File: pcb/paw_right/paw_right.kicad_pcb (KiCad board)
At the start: 2 copper layers, 141.8 x 96 mm, 44 parts, among them U1 Nice_Nano_V2

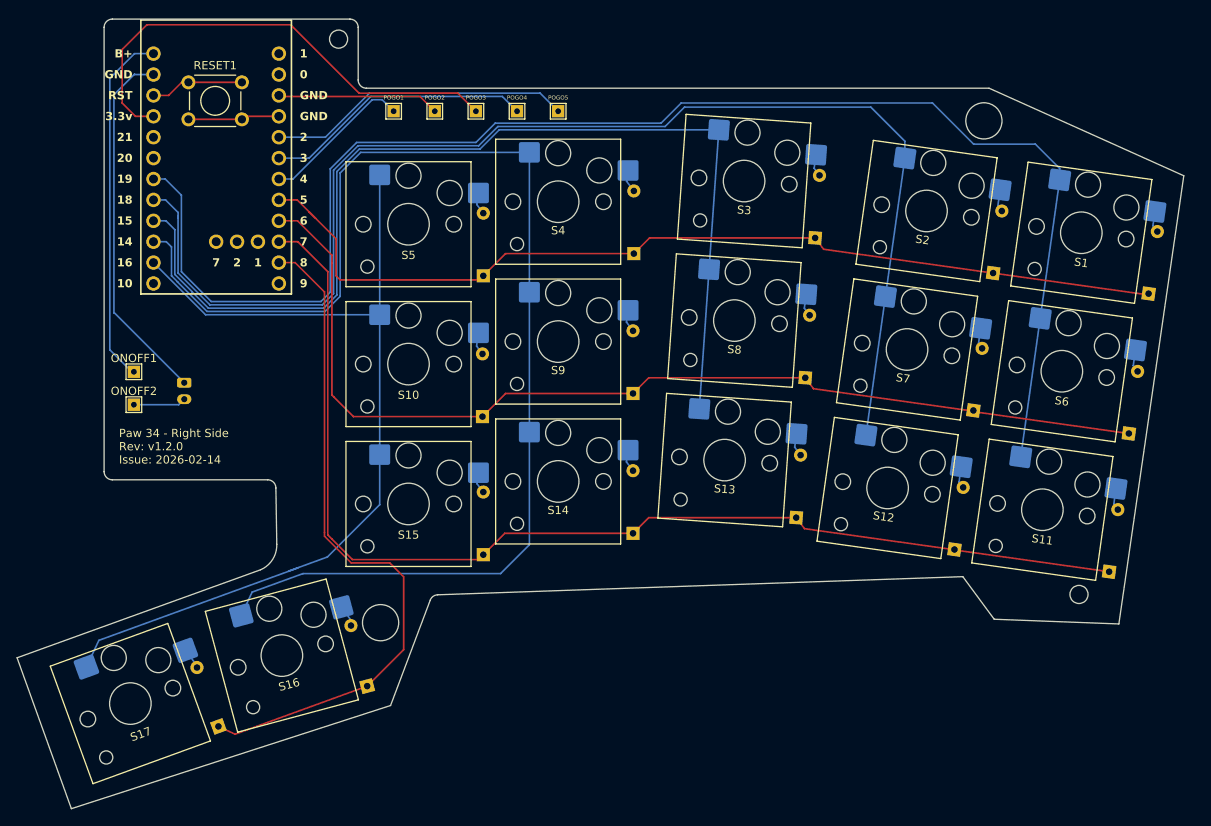
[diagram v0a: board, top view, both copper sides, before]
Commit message: PCB rev 1.2.0
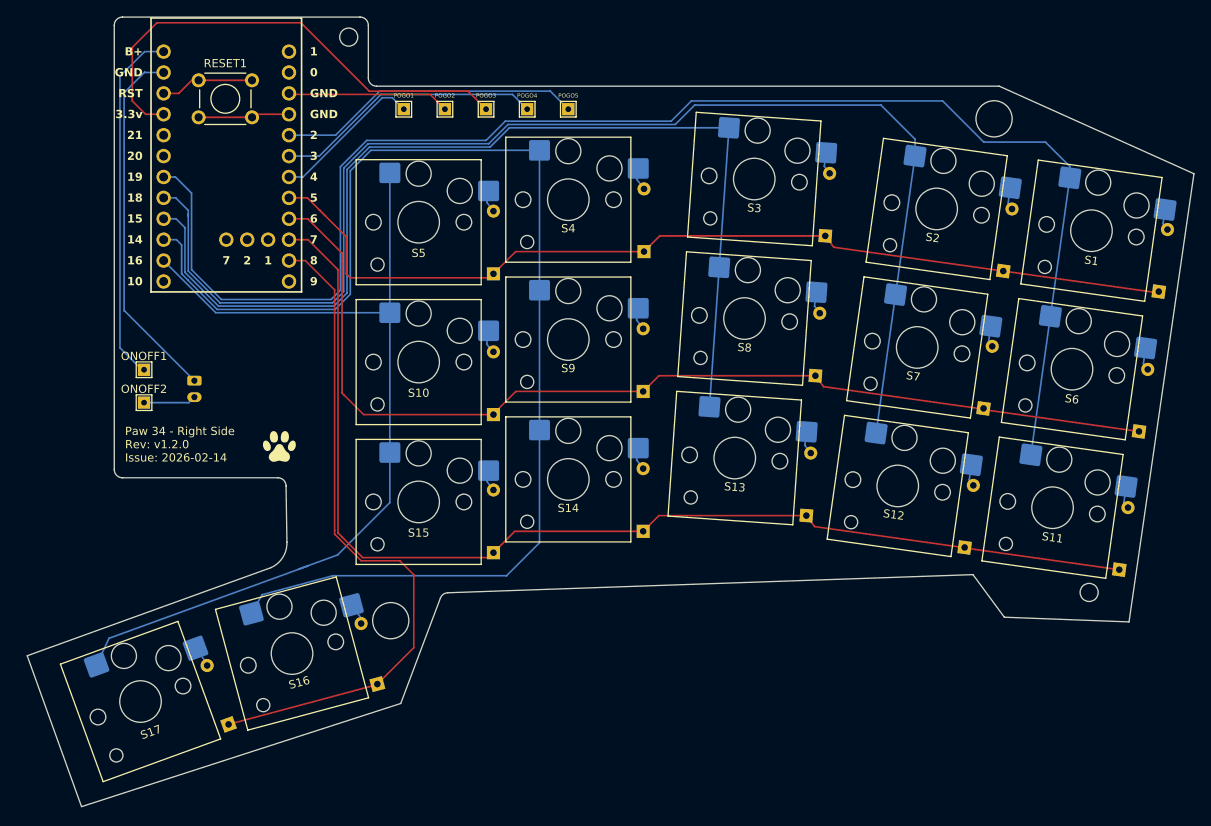
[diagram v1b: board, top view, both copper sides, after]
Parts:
- added G***: LOGO, MentalDesk:Paw_Logo, F.Cu at (108.3, 175.3)
- moved D10 1.36 mm to (134.3, 171.5)
- moved D9 1.26 mm to (152.5, 168.7)
- moved D4 1.26 mm to (152.6, 151.7)
- moved S13 1.26 mm to (163.6, 176.8)
- moved S16 1.26 mm to (109.8, 200.5)
- moved D15 1.26 mm to (134.3, 188.3)
- moved D3 1.26 mm to (174.6, 149.8)
- moved D7 1.26 mm to (193.9, 170.7)
- moved D12 1.26 mm to (191.6, 187.6)
- moved S5 1.26 mm to (125.2, 148.1)
- moved S11 1.26 mm to (202.3, 182.8)
- moved ONOFF1 1.26 mm to (91.8, 166.0)
- moved D2 1.26 mm to (196.3, 154.0)
- moved RESET1 1.26 mm to (98.5, 130.8)
- moved S17 1.26 mm to (91.4, 206.3)
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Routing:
- net Row 3: track 82.8 -> 82.3 mm
